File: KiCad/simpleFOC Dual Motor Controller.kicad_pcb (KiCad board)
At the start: 4 copper layers, 50 x 50 mm, 41 parts, among them Q301 MS6001Y, Q302 MS6001Y, Q401 MS6001Y, Q402 MS6001Y, Q501 MS6001Y, Q502 MS6001Y, Q701 MS6001Y, Q702 MS6001Y, Q801 MS6001Y, Q802 MS6001Y, Q901 MS6001Y, Q902 MS6001Y, U101 STM32F103C8Tx, U201 DRV8323HRTAT, U601 DRV8323HRTAT

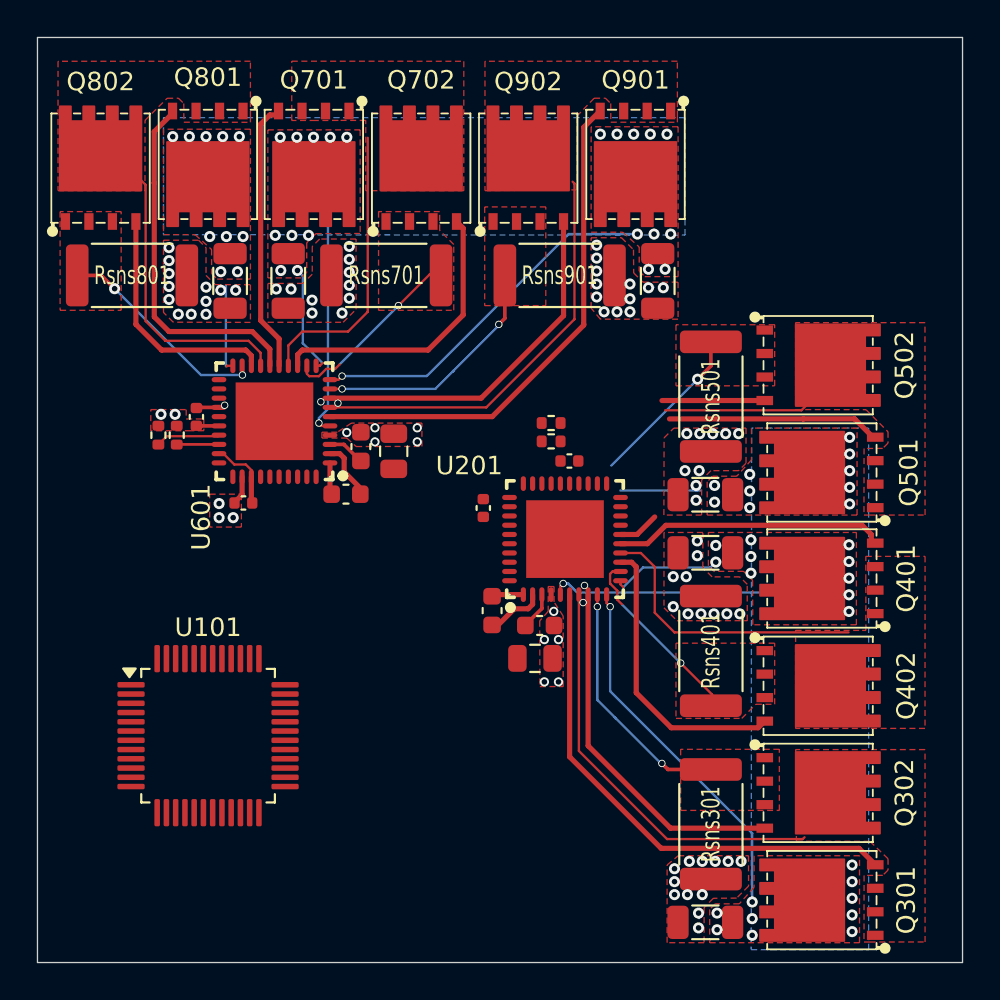
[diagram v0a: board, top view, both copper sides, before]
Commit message: started adding supporting components
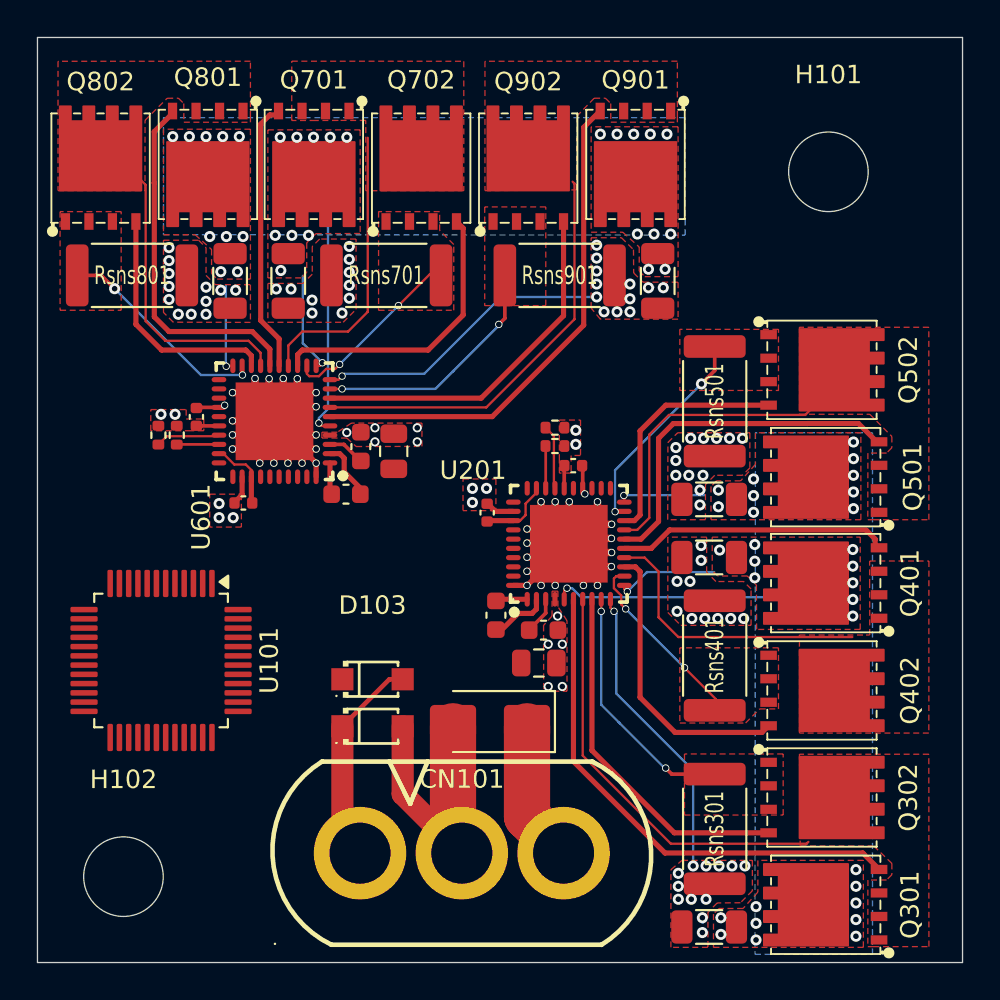
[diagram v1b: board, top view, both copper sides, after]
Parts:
- added CN101: MR60-F, easyeda2kicad:CONN-TH_3P-P5.50_MR60-F, F.Cu at (122.9, 69.1)
- added D101: SMAJ36A, Diode_SMD:D_SMA, F.Cu at (124.5, 62.0)
- added D103: DSK26_C7502712, easyeda2kicad:SOD-123FL_L2.7-W1.8-LS3.8-RD, F.Cu at (118.1, 59.7)
- added D104: SMF5.0A_C19077497, easyeda2kicad:SOD-123FL_L2.7-W1.8-LS3.8-RD, F.Cu at (118.1, 62.2)
- added H101: MountingHole, MountingHole:MountingHole_4.3mm_M4, F.Cu at (142.8, 32.3)
- added H102: MountingHole, MountingHole:MountingHole_4.3mm_M4, F.Cu at (104.6, 70.4)
- moved U101 4.79 mm to (106.7, 58.7), turned to -90 degrees
- moved Q502 0.33 mm to (141.3, 43.0)
- moved Rsns401 0.33 mm to (136.6, 58.4)
- moved U201 0.33 mm to (128.7, 52.4)
- moved C201 0.33 mm to (127.1, 58.8)
- moved C205 0.33 mm to (129.0, 48.1)
- moved Q402 0.33 mm to (141.3, 60.3)
- moved Rsns501 0.33 mm to (136.6, 44.7)
- moved C202 0.33 mm to (127.4, 57.0)
- moved Q302 0.33 mm to (141.3, 66.1)
- moved Rsns301 0.33 mm to (136.6, 67.8)
- moved C203 0.33 mm to (124.8, 56.2)
- moved C204 0.33 mm to (124.3, 50.7)
- moved R201 0.33 mm to (128.0, 46.1)
- moved R202 0.33 mm to (128.0, 47.1)
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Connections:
- C601 pad 1: /Motor Driver 2/Motor_VIN -> /Motor Driver 1/Motor_VIN
- C602 pad 1: /Motor Driver 2/Motor_VIN -> /Motor Driver 1/Motor_VIN
- C701 pad 1: /Motor Driver 2/Motor_VIN -> /Motor Driver 1/Motor_VIN
- C801 pad 1: /Motor Driver 2/Motor_VIN -> /Motor Driver 1/Motor_VIN
- C901 pad 1: /Motor Driver 2/Motor_VIN -> /Motor Driver 1/Motor_VIN
- Q701 pad 5: /Motor Driver 2/Motor_VIN -> /Motor Driver 1/Motor_VIN
- Q801 pad 5: /Motor Driver 2/Motor_VIN -> /Motor Driver 1/Motor_VIN
- Q901 pad 5: /Motor Driver 2/Motor_VIN -> /Motor Driver 1/Motor_VIN
- U101 pad 1: unconnected-(U101-VBAT-Pad1) -> +3.3V
- U101 pad 23: Net-(U101-VSS-Pad23) -> GND
- U101 pad 24: unconnected-(U101-VDD-Pad24) -> +3.3V
- U101 pad 35: Net-(U101-VSS-Pad23) -> GND
- U101 pad 36: unconnected-(U101-VDD-Pad36) -> +3.3V
- U101 pad 47: Net-(U101-VSS-Pad23) -> GND
- U101 pad 48: unconnected-(U101-VDD-Pad48) -> +3.3V
- U101 pad 8: unconnected-(U101-VSSA-Pad8) -> GND
- U101 pad 9: unconnected-(U101-VDDA-Pad9) -> +3.3V
- U601 pad 4: /Motor Driver 2/Motor_VIN -> /Motor Driver 1/Motor_VIN
- U601 pad 5: /Motor Driver 2/Motor_VIN -> /Motor Driver 1/Motor_VIN
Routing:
- net GND: track 53.8 -> 139.6 mm, vias 74 -> 117
- net /Motor Driver 2/Motor_VIN: track 20.2 -> 0.00 mm, vias 36 -> 0
- net /Motor Driver 1/Motor_VIN: track 20.2 -> 36.9 mm, vias 36 -> 71
- net Net-(D103-A): track 0.00 -> 11.6 mm
- net /Motor Driver 1/Pole 3/GL: track 5.63 -> 12.9 mm
- net /Motor Driver 1/Pole 3/PoleOut: track 10.5 -> 17.3 mm
- net /Motor Driver 1/Pole 3/GH: track 13.6 -> 19.3 mm
- net /Motor Driver 1/DVDD: track 0.00 -> 3.61 mm
- net Net-(U201-IDRIVE): track 0.00 -> 3.40 mm
- net /Motor Driver 1/Pole 3/SP: track 8.92 -> 11.7 mm, vias 1 -> 2
- net Net-(U201-VDS): track 0.00 -> 2.44 mm
- net /Motor Driver 1/VREF: track 0.00 -> 0.98 mm, vias 0 -> 1
- net /Motor Driver 2/Pole 3/PoleOut: track 18.1 -> 17.3 mm
- removed copper zone on B.Cu, net /Motor Driver 2/Motor_VIN
- removed copper zone on F.Cu, net /Motor Driver 2/Motor_VIN
